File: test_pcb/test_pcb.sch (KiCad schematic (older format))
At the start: 70 parts, among them K0 KEYSW, K1 KEYSW, K10 KEYSW, K12 KEYSW, K13 KEYSW, K14 KEYSW, K15 KEYSW, K16 KEYSW, K17 KEYSW, K18 KEYSW, K2 KEYSW, K20 KEYSW, K21 KEYSW, K22 KEYSW, K3 KEYSW, K4 KEYSW, K5 KEYSW, K6 KEYSW, K7 KEYSW, K8 KEYSW, K9 KEYSW, P1 CONN_01X08, P2 CONN_01X08, P3 CONN_01X06, U1 STP16CP05

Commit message: test pcb seem to have fixed the routing bug
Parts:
- added JP1, JP4: Jumper_NC_Small, Pin_Headers:Pin_Header_Angled_1x02_Pitch1.27mm, symbol Jumper_NC_Small
- added JP2, JP3, JP5: Jumper_NC_Dual, Pin_Headers:Pin_Header_Angled_1x03_Pitch1.27mm, symbol Jumper_NC_Dual
- P1: value CONN_01X08 -> CONN_01X10; footprint Socket_Strips:Socket_Strip_Straight_1x08_Pitch2.54mm -> Socket_Strips:Socket_Strip_Straight_1x10_Pitch2.54mm; symbol CONN_01X08 -> CONN_01X10
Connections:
- wire segments 242 -> 254
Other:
- moved on the sheet: R0, R2

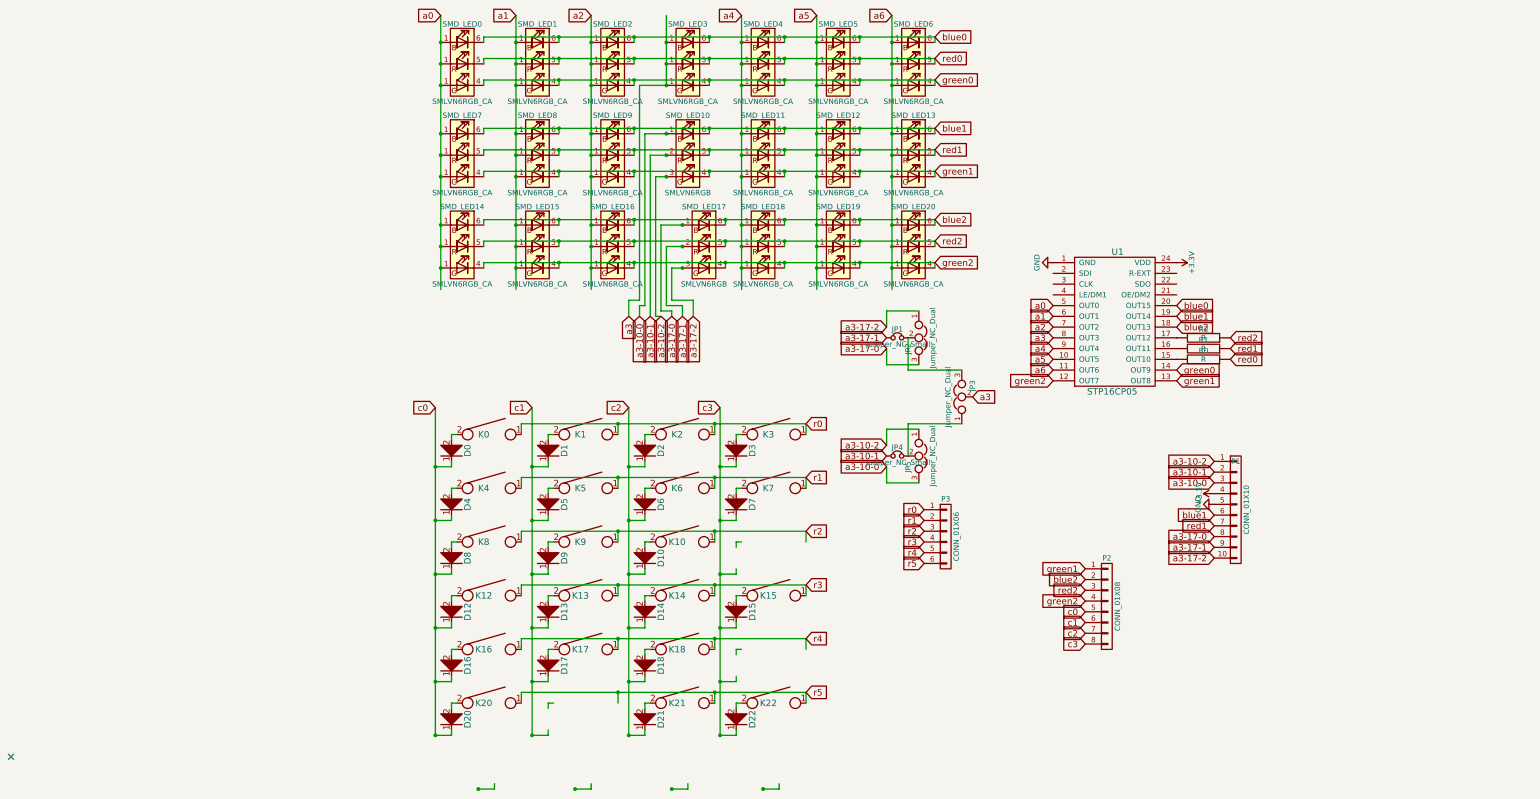
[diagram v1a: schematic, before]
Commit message: testp progress
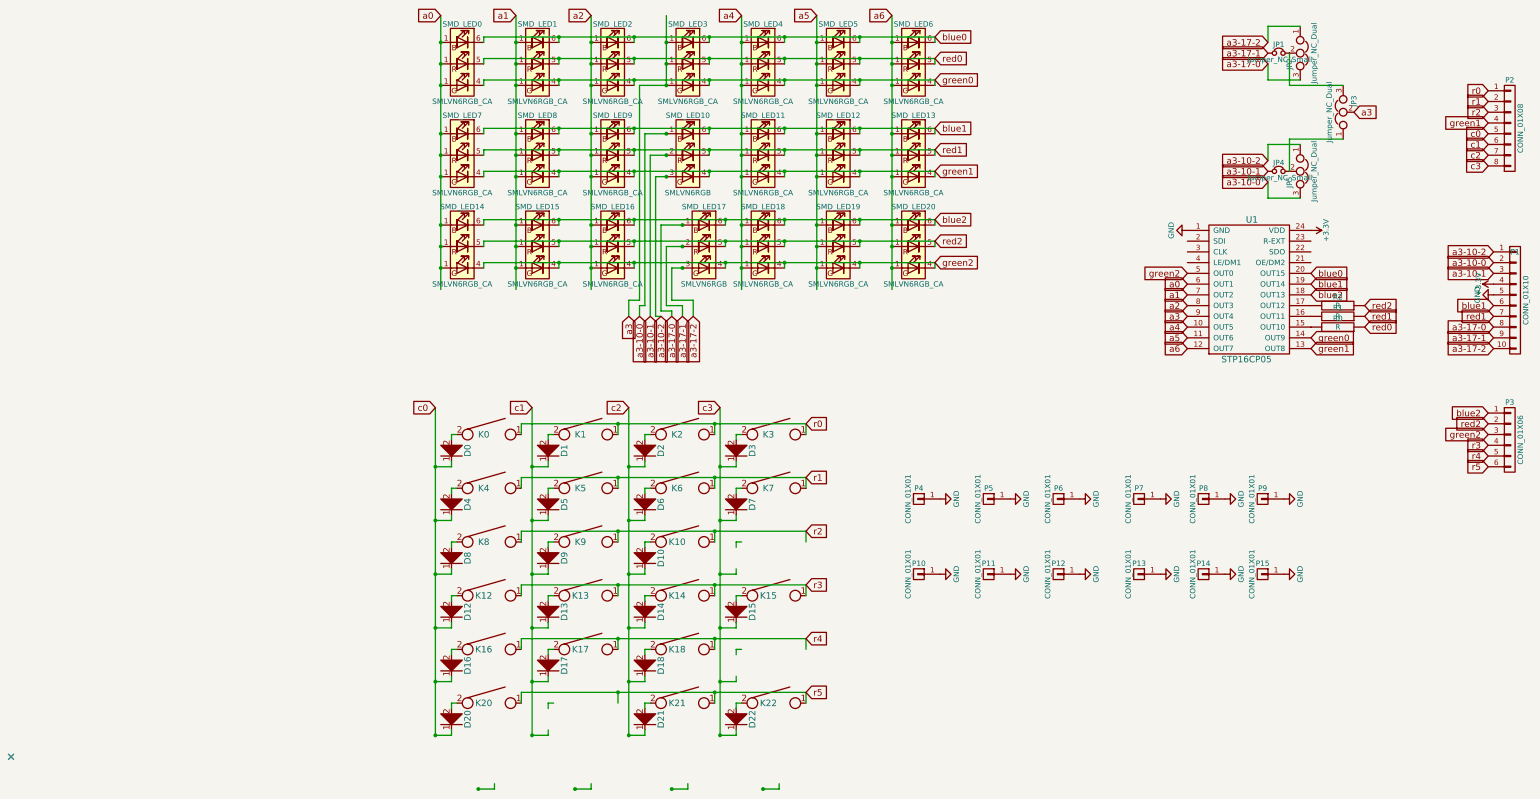
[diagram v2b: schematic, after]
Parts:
- added P10, P11, P12, P13, P14, P15, P4, P5, P6, P7, P8, P9: CONN_01X01, Socket_Strips:Socket_Strip_Straight_1x01_Pitch1.27mm, symbol CONN_01X01
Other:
- moved on the sheet: JP1, JP2, JP3, JP4, JP5, P1, P2, P3, R0, R1, R2, U1

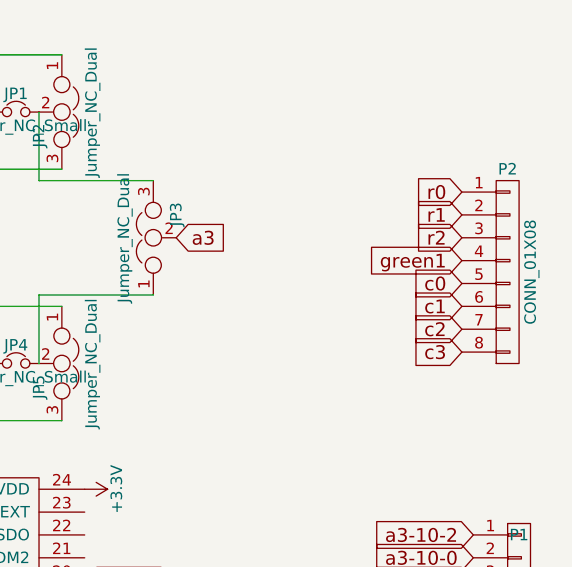
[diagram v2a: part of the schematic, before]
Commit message: test a bit better
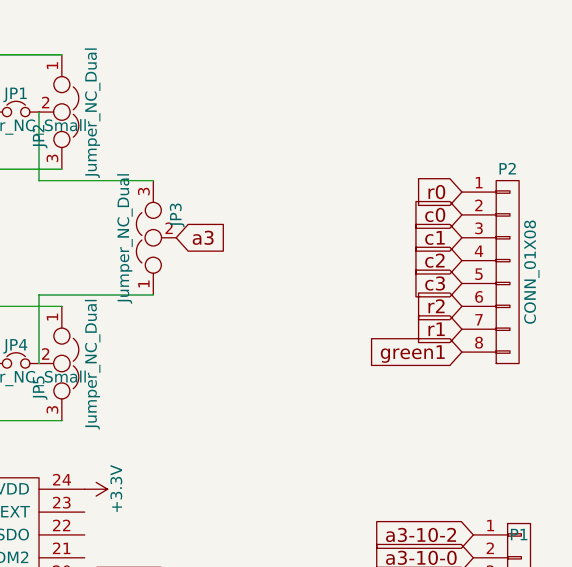
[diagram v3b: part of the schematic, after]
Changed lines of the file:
@@
 a3-17-2
 $Comp
-L GND #PWR1
+L GND #PWR01
 U 1 1 58A5AE89
 P 7750 2550
-F 0 "#PWR1" H 7750 2300 50  0001 C CNN
+F 0 "#PWR01" H 7750 2300 50  0001 C CNN
 F 1 "GND" H 7750 2400 50  0000 C CNN
 F 2 "" H 7750 2550 50  0000 C CNN
@@
 a3-17-2
 $Comp
-L +3.3V #PWR2
+L +3.3V #PWR02
 U 1 1 58A3C033
 P 8900 2550
-F 0 "#PWR2" H 8900 2400 50  0001 C CNN
+F 0 "#PWR02" H 8900 2400 50  0001 C CNN
 F 1 "+3.3V" H 8900 2690 50  0000 C CNN
 F 2 "" H 8900 2550 50  0000 C CNN
@@
 Text GLabel 10600 3350 0    60   Input ~ 0
 red1
-Text GLabel 10550 1550 0    60   Input ~ 0
+Text GLabel 10550 1950 0    60   Input ~ 0
 green1
 Text GLabel 10550 4250 0    60   Input ~ 0
@@
 	1    0    0    -1
 $EndComp
+Text GLabel 10550 1350 0    60   Input ~ 0
+c0
+Text GLabel 10550 1450 0    60   Input ~ 0
+c1
+Text GLabel 10550 1550 0    60   Input ~ 0
+c2
 Text GLabel 10550 1650 0    60   Input ~ 0
-c0
-Text GLabel 10550 1750 0    60   Input ~ 0
-c1
-Text GLabel 10550 1850 0    60   Input ~ 0
-c2
-Text GLabel 10550 1950 0    60   Input ~ 0
 c3
 Text GLabel 10550 1250 0    60   Input ~ 0
 r0
-Text GLabel 10550 1350 0    60   Input ~ 0
+Text GLabel 10550 1850 0    60   Input ~ 0
 r1
-Text GLabel 10550 1450 0    60   Input ~ 0
+Text GLabel 10550 1750 0    60   Input ~ 0
 r2
 Text GLabel 10550 4550 0    60   Input ~ 0
@@
 $EndComp
 $Comp
-L GND #PWR4
+L GND #PWR03
 U 1 1 58BA412A
 P 10600 3150
-F 0 "#PWR4" H 10600 2900 50  0001 C CNN
+F 0 "#PWR03" H 10600 2900 50  0001 C CNN
 F 1 "GND" H 10600 3000 50  0000 C CNN
 F 2 "" H 10600 3150 50  0000 C CNN
@@
 $EndComp
 $Comp
-L +3.3V #PWR3
+L +3.3V #PWR04
 U 1 1 58BA41CE
 P 10600 3050
-F 0 "#PWR3" H 10600 2900 50  0001 C CNN
+F 0 "#PWR04" H 10600 2900 50  0001 C CNN
 F 1 "+3.3V" H 10600 3190 50  0000 C CNN
 F 2 "" H 10600 3050 50  0000 C CNN
@@
 $EndComp
 $Comp
-L GND #PWR5
+L GND #PWR05
 U 1 1 58BABD17
 P 5450 5050
-F 0 "#PWR5" H 5450 4800 50  0001 C CNN
+F 0 "#PWR05" H 5450 4800 50  0001 C CNN
 F 1 "GND" H 5450 4900 50  0000 C CNN
 F 2 "" H 5450 5050 50  0000 C CNN
@@
 $EndComp
 $Comp
-L GND #PWR6
+L GND #PWR06
 U 1 1 58BACEDF
 P 6100 5050
-F 0 "#PWR6" H 6100 4800 50  0001 C CNN
+F 0 "#PWR06" H 6100 4800 50  0001 C CNN
 F 1 "GND" H 6100 4900 50  0000 C CNN
 F 2 "" H 6100 5050 50  0000 C CNN
@@
 $EndComp
 $Comp
-L GND #PWR8
+L GND #PWR07
 U 1 1 58BAD6B9
 P 7500 5050
-F 0 "#PWR8" H 7500 4800 50  0001 C CNN
+F 0 "#PWR07" H 7500 4800 50  0001 C CNN
 F 1 "GND" H 7500 4900 50  0000 C CNN
 F 2 "" H 7500 5050 50  0000 C CNN
@@
 $EndComp
 $Comp
-L GND #PWR7
+L GND #PWR08
 U 1 1 58BAEE31
 P 6750 5050
-F 0 "#PWR7" H 6750 4800 50  0001 C CNN
+F 0 "#PWR08" H 6750 4800 50  0001 C CNN
 F 1 "GND" H 6750 4900 50  0000 C CNN
 F 2 "" H 6750 5050 50  0000 C CNN
@@
 $EndComp
 $Comp
-L GND #PWR10
+L GND #PWR09
 U 1 1 58BAEE3D
 P 8650 5050
-F 0 "#PWR10" H 8650 4800 50  0001 C CNN
+F 0 "#PWR09" H 8650 4800 50  0001 C CNN
 F 1 "GND" H 8650 4900 50  0000 C CNN
 F 2 "" H 8650 5050 50  0000 C CNN
@@
 $EndComp
 $Comp
-L GND #PWR9
+L GND #PWR010
 U 1 1 58BAEE49
 P 8100 5050
-F 0 "#PWR9" H 8100 4800 50  0001 C CNN
+F 0 "#PWR010" H 8100 4800 50  0001 C CNN
 F 1 "GND" H 8100 4900 50  0000 C CNN
 F 2 "" H 8100 5050 50  0000 C CNN
@@
 $EndComp
 $Comp
-L GND #PWR11
+L GND #PWR011
 U 1 1 58BB11B2
 P 5450 5750
-F 0 "#PWR11" H 5450 5500 50  0001 C CNN
+F 0 "#PWR011" H 5450 5500 50  0001 C CNN
 F 1 "GND" H 5450 5600 50  0000 C CNN
 F 2 "" H 5450 5750 50  0000 C CNN
@@
 $EndComp
 $Comp
-L GND #PWR12
+L GND #PWR012
 U 1 1 58BB11BE
 P 6100 5750
-F 0 "#PWR12" H 6100 5500 50  0001 C CNN
+F 0 "#PWR012" H 6100 5500 50  0001 C CNN
 F 1 "GND" H 6100 5600 50  0000 C CNN
 F 2 "" H 6100 5750 50  0000 C CNN
@@
 $EndComp
 $Comp
-L GND #PWR14
+L GND #PWR013
 U 1 1 58BB11CA
 P 7500 5750
-F 0 "#PWR14" H 7500 5500 50  0001 C CNN
+F 0 "#PWR013" H 7500 5500 50  0001 C CNN
 F 1 "GND" H 7500 5600 50  0000 C CNN
 F 2 "" H 7500 5750 50  0000 C CNN
@@
 $EndComp
 $Comp
-L GND #PWR13
+L GND #PWR014
 U 1 1 58BB11D6
 P 6750 5750
-F 0 "#PWR13" H 6750 5500 50  0001 C CNN
+F 0 "#PWR014" H 6750 5500 50  0001 C CNN
 F 1 "GND" H 6750 5600 50  0000 C CNN
 F 2 "" H 6750 5750 50  0000 C CNN
@@
 $EndComp
 $Comp
-L GND #PWR16
+L GND #PWR015
 U 1 1 58BB11E2
 P 8650 5750
-F 0 "#PWR16" H 8650 5500 50  0001 C CNN
+F 0 "#PWR015" H 8650 5500 50  0001 C CNN
 F 1 "GND" H 8650 5600 50  0000 C CNN
 F 2 "" H 8650 5750 50  0000 C CNN
@@
 $EndComp
 $Comp
-L GND #PWR15
+L GND #PWR016
 U 1 1 58BB11EE
 P 8100 5750
-F 0 "#PWR15" H 8100 5500 50  0001 C CNN
+F 0 "#PWR016" H 8100 5500 50  0001 C CNN
 F 1 "GND" H 8100 5600 50  0000 C CNN
 F 2 "" H 8100 5750 50  0000 C CNN
